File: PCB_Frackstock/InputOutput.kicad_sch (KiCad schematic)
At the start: 30 parts, among them J1 87224-3, U11 CC1101RGPR, U7 BMI323, Y2 26MHz

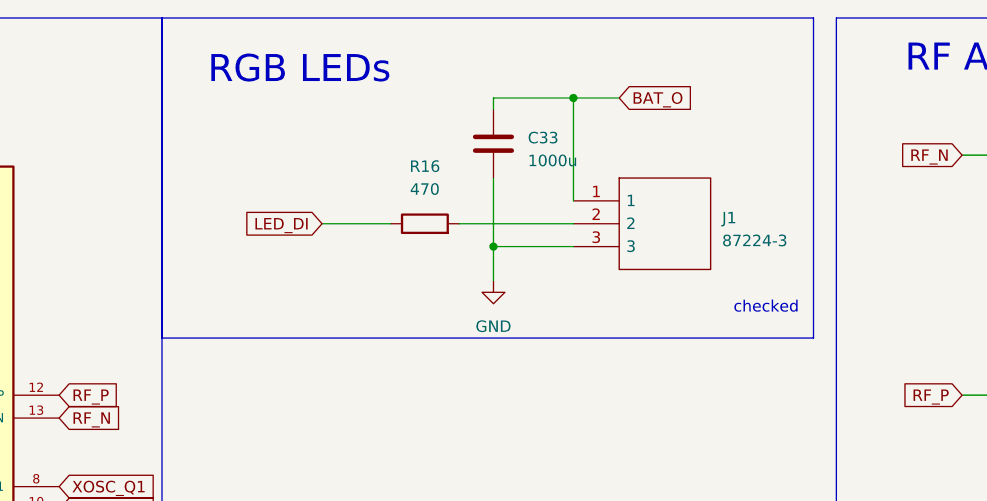
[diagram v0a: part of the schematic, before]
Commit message: Schema_fertig
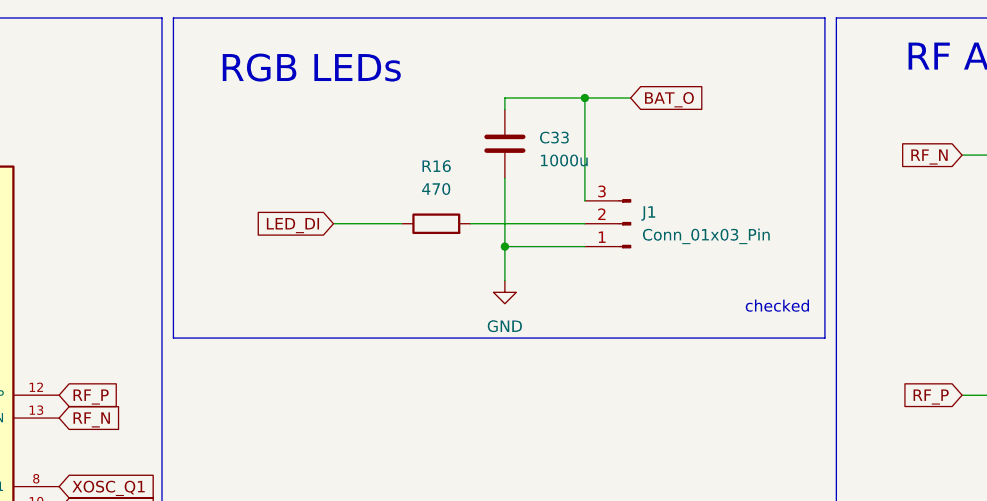
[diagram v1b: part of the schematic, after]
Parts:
- removed J1: 87224-3, KiCad:872243, symbol 87224-3:87224-3
- added J1: Conn_01x03_Pin, Connector_PinHeader_2.54mm:PinHeader_1x03_P2.54mm_Vertical, symbol Connector:Conn_01x03_Pin
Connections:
- net BAT_O: now also J1.3 (Pin_3)
- net GND: now also J1.1 (Pin_1)
- net at R16.2: now also J1.2 (Pin_2)
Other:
- moved on the sheet: C33, R16

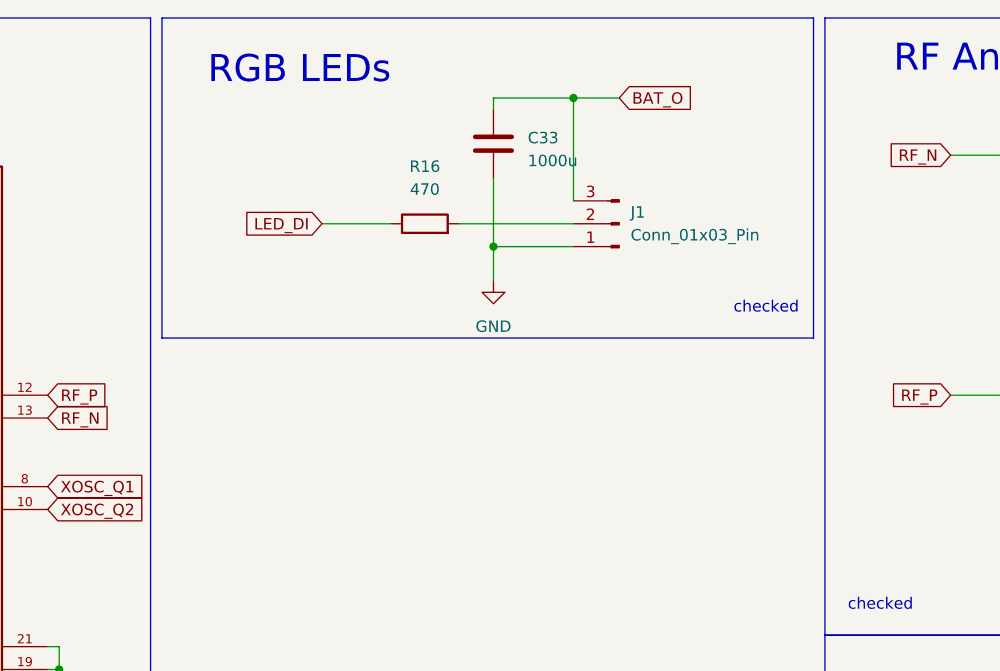
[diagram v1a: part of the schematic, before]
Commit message: Layout Fertig
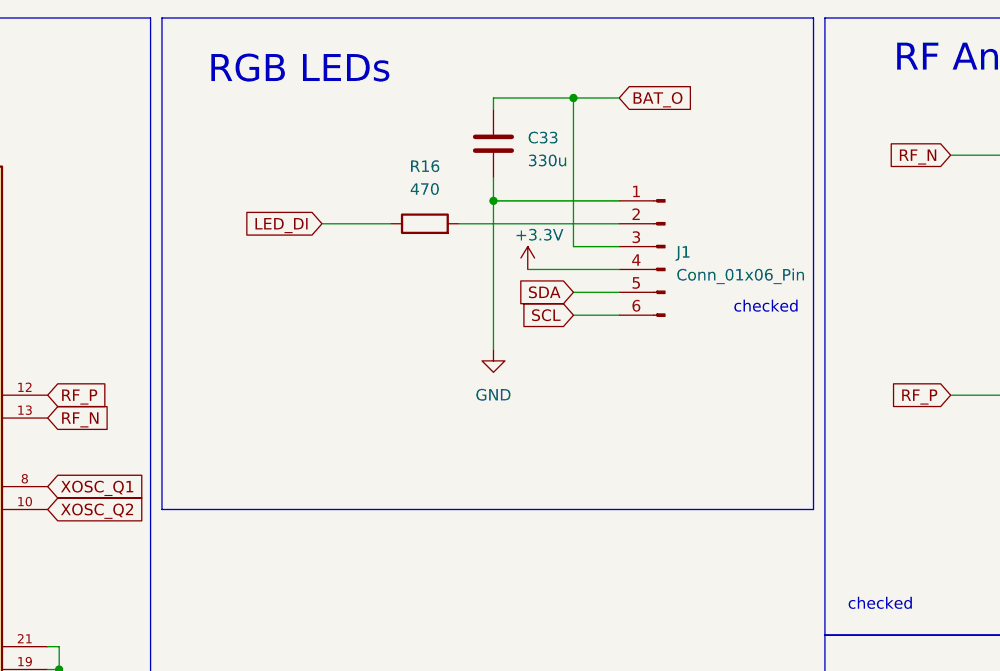
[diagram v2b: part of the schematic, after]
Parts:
- removed J1: Conn_01x03_Pin, Connector_PinHeader_2.54mm:PinHeader_1x03_P2.54mm_Vertical, symbol Connector:Conn_01x03_Pin
- added J1: Conn_01x06_Pin, symbol Connector:Conn_01x06_Pin
- C33: value 1000u -> 330u; footprint Capacitor_SMD:CP_Elec_8x10.5 -> Capacitor_SMD:C_0805_2012Metric_Pad1.18x1.45mm_HandSolder
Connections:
- net +3.3V: now also J1.4 (Pin_4)
- net BAT_O: now also J1.3 (Pin_3)
- net GND: now also J1.1 (Pin_1)
- net at R16.2: now also J1.2 (Pin_2)
- new net SCL: J1.6 (Pin_6)
- new net SDA: J1.5 (Pin_5)
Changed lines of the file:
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@@
   (junction (at 228.6 97.79) (diameter 0) (color 0 0 0 0)
   )
+  (junction (at 134.62 34.29) (diameter 0) (color 0 0 0 0)
+  )
   (junction (at 83.82 177.8) (diameter 0) (color 0 0 0 0)
   )
-  (junction (at 134.62 39.37) (diameter 0) (color 0 0 0 0)
-  )
   (junction (at 240.03 107.95) (diameter 0) (color 0 0 0 0)
   )
@@
     (stroke (width 0) (type default))
   )
+  (wire (pts (xy 143.51 46.99) (xy 148.59 46.99))
+    (stroke (width 0) (type default))
+  )
   (wire (pts (xy 38.1 40.64) (xy 38.1 38.1))
     (stroke (width 0) (type default))
@@
     (stroke (width 0) (type default))
   )
+  (wire (pts (xy 134.62 34.29) (xy 148.59 34.29))
+    (stroke (width 0) (type default))
+  )
+  (wire (pts (xy 134.62 34.29) (xy 134.62 50.8))
+    (stroke (width 0) (type default))
+  )
   (wire (pts (xy 185.42 55.88) (xy 194.31 55.88))
     (stroke (width 0) (type default))
   )
-  (wire (pts (xy 134.62 31.75) (xy 134.62 39.37))
-    (stroke (width 0) (type default))
-  )
   (wire (pts (xy 232.41 41.91) (xy 237.49 41.91))
     (stroke (width 0) (type default))
@@
     (stroke (width 0) (type default))
   )
+  (wire (pts (xy 138.43 41.91) (xy 148.59 41.91))
+    (stroke (width 0) (type default))
+  )
   (wire (pts (xy 134.62 22.86) (xy 134.62 24.13))
     (stroke (width 0) (type default))
@@
     (stroke (width 0) (type default))
   )
-  (wire (pts (xy 130.81 36.83) (xy 143.51 36.83))
+  (wire (pts (xy 130.81 36.83) (xy 148.59 36.83))
     (stroke (width 0) (type default))
   )
@@
     (stroke (width 0) (type default))
   )
-  (wire (pts (xy 134.62 39.37) (xy 134.62 43.18))
+  (wire (pts (xy 134.62 31.75) (xy 134.62 34.29))
     (stroke (width 0) (type default))
   )
@@
     (stroke (width 0) (type default))
   )
+  (wire (pts (xy 143.51 44.45) (xy 148.59 44.45))
+    (stroke (width 0) (type default))
+  )
   (wire (pts (xy 251.46 97.79) (xy 251.46 99.06))
     (stroke (width 0) (type default))
@@
     (stroke (width 0) (type default))
   )
-  (wire (pts (xy 143.51 22.86) (xy 143.51 34.29))
+  (wire (pts (xy 143.51 22.86) (xy 143.51 39.37))
+    (stroke (width 0) (type default))
+  )
+  (wire (pts (xy 143.51 39.37) (xy 148.59 39.37))
     (stroke (width 0) (type default))
   )
@@
     (stroke (width 0) (type default))
   )
-  (wire (pts (xy 134.62 39.37) (xy 143.51 39.37))
-    (stroke (width 0) (type default))
-  )
   (wire (pts (xy 232.41 55.88) (xy 228.6 55.88))
     (stroke (width 0) (type default))
@@
     (stroke (width 0) (type default))
   )
-  (rectangle (start 97.79 13.97) (end 170.18 49.53)
+  (rectangle (start 97.79 13.97) (end 170.18 68.58)
     (stroke (width 0) (type default))
     (fill (type none))
@@
     )
   )
+  (global_label "SDA" (shape input) (at 143.51 44.45 180) (fields_autoplaced)
+    (effects (font (size 1.27 1.27)) (justify right))
+    (property "Intersheetrefs" "${INTERSHEET_REFS}" (at 137.0361 44.45 0)
+      (effects (font (size 1.27 1.27)) (justify right) hide)
+    )
+  )
   (global_label "RF_P" (shape input) (at 185.42 55.88 180) (fields_autoplaced)
     (effects (font (size 1.27 1.27)) (justify right))
@@
     )
   )
+  (global_label "SCL" (shape input) (at 143.51 46.99 180) (fields_autoplaced)
+    (effects (font (size 1.27 1.27)) (justify right))
+    (property "Intersheetrefs" "${INTERSHEET_REFS}" (at 137.0966 46.99 0)
+      (effects (font (size 1.27 1.27)) (justify right) hide)
+    )
+  )
   (global_label "XOSC_Q2" (shape input) (at 85.09 68.58 0) (fields_autoplaced)
     (effects (font (size 1.27 1.27)) (justify left))
@@
         (path "/d92252e1-c687-49e6-87c8-e9430a2c933e/c15a2309-71af-495b-84ee-43442cf95a1c"
           (reference "#PWR019") (unit 1)
+        )
+      )
+    )
+  )
+  (symbol (lib_id "power:+3.3V") (at 138.43 41.91 0) (unit 1)
+    (in_bom yes) (on_board yes) (dnp no)
+    (property "Reference" "#PWR03" (at 138.43 45.72 0)
+      (effects (font (size 1.27 1.27)) hide)
+    )
+    (property "Value" "+3.3V" (at 139.7 38.1 0)
+      (effects (font (size 1.27 1.27)))
+    )
+    (property "Footprint" "" (at 138.43 41.91 0)
+      (effects (font (size 1.27 1.27)) hide)
+    )
+    (property "Datasheet" "" (at 138.43 41.91 0)
+      (effects (font (size 1.27 1.27)) hide)
+    )
+    (pin "1")
+    (instances
+      (project "Frackstock"
+        (path "/d92252e1-c687-49e6-87c8-e9430a2c933e/c15a2309-71af-495b-84ee-43442cf95a1c"
+          (reference "#PWR03") (unit 1)
         )
       )
@@
     )
   )
-  (symbol (lib_id "power:GND") (at 134.62 43.18 0) (unit 1)
-    (in_bom yes) (on_board yes) (dnp no) (fields_autoplaced)
-    (property "Reference" "#PWR013" (at 134.62 49.53 0)
-      (effects (font (size 1.27 1.27)) hide)
-    )
-    (property "Value" "GND" (at 134.62 48.26 0)
-      (effects (font (size 1.27 1.27)))
-    )
-    (property "Footprint" "" (at 134.62 43.18 0)
-      (effects (font (size 1.27 1.27)) hide)
-    )
-    (property "Datasheet" "" (at 134.62 43.18 0)
+  (symbol (lib_id "power:GND") (at 134.62 50.8 0) (unit 1)
+    (in_bom yes) (on_board yes) (dnp no) (fields_autoplaced)
+    (property "Reference" "#PWR013" (at 134.62 57.15 0)
+      (effects (font (size 1.27 1.27)) hide)
+    )
+    (property "Value" "GND" (at 134.62 55.88 0)
+      (effects (font (size 1.27 1.27)))
+    )
+    (property "Footprint" "" (at 134.62 50.8 0)
+      (effects (font (size 1.27 1.27)) hide)
+    )
+    (property "Datasheet" "" (at 134.62 50.8 0)
       (effects (font (size 1.27 1.27)) hide)
     )
@@
       (effects (font (size 1.27 1.27)) (justify right))
     )
-    (property "Value" "1000u" (at 138.43 29.845 0)
+    (property "Value" "330u" (at 138.43 29.845 0)
       (effects (font (size 1.27 1.27)) (justify right))
     )
-    (property "Footprint" "Capacitor_SMD:CP_Elec_8x10.5" (at 133.6548 24.13 0)
+    (property "Footprint" "Capacitor_SMD:C_0805_2012Metric_Pad1.18x1.45mm_HandSolder" (at 133.6548 24.13 0)
       (effects (font (size 1.27 1.27)) hide)
     )
@@
         (path "/d92252e1-c687-49e6-87c8-e9430a2c933e/c15a2309-71af-495b-84ee-43442cf95a1c"
           (reference "C37") (unit 1)
+        )
+      )
+    )
+  )
+  (symbol (lib_id "Connector:Conn_01x06_Pin") (at 153.67 39.37 0) (mirror y) (unit 1)
+    (in_bom yes) (on_board yes) (dnp no) (fields_autoplaced)
+    (property "Reference" "J1" (at 154.94 40.005 0)
+      (effects (font (size 1.27 1.27)) (justify right))
+    )
+    (property "Value" "Conn_01x06_Pin" (at 154.94 42.545 0)
+      (effects (font (size 1.27 1.27)) (justify right))
+    )
+    (property "Footprint" "" (at 153.67 39.37 0)
+      (effects (font (size 1.27 1.27)) hide)
+    )
+    (property "Datasheet" "~" (at 153.67 39.37 0)
+      (effects (font (size 1.27 1.27)) hide)
+    )
+    (pin "1")
+    (pin "2")
+    (pin "3")
+    (pin "4")
+    (pin "5")
+    (pin "6")
+    (instances
+      (project "Frackstock"
+        (path "/d92252e1-c687-49e6-87c8-e9430a2c933e/c15a2309-71af-495b-84ee-43442cf95a1c"
+          (reference "J1") (unit 1)
         )
       )
@@
         )
       )
-    )
-  )
-  (symbol (lib_id "Connector:Conn_01x03_Pin") (at 148.59 36.83 180) (unit 1)
-    (in_bom yes) (on_board yes) (dnp no) (fields_autoplaced)
-    (property "Reference" "J1" (at 149.86 35.56 0)
-      (effects (font (size 1.27 1.27)) (justify right))
-    )
-    (property "Value" "Conn_01x03_Pin" (at 149.86 38.1 0)
-      (effects (font (size 1.27 1.27)) (justify right))
-    )
-    (property "Footprint" "Connector_PinHeader_2.54mm:PinHeader_1x03_P2.54mm_Vertical" (at 148.59 36.83 0)
-      (effects (font (size 1.27 1.27)) hide)
-    )
-    (property "Datasheet" "~" (at 148.59 36.83 0)
-      (effects (font (size 1.27 1.27)) hide)
-    )
-    (pin "1")
-    (pin "2")
-    (pin "3")
-    (instances
-      (project "Frackstock"
-        (path "/d92252e1-c687-49e6-87c8-e9430a2c933e/c15a2309-71af-495b-84ee-43442cf95a1c"
-          (reference "J1") (unit 1)
-        )
-      )

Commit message: Layout Update
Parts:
- J1: footprint (none) -> Frack:PinHeader_2x03_P2.54mm_Vertical_SMD_kleiner
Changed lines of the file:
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@@
       (effects (font (size 1.27 1.27)) (justify right))
     )
-    (property "Footprint" "" (at 153.67 39.37 0)
+    (property "Footprint" "Frack:PinHeader_2x03_P2.54mm_Vertical_SMD_kleiner" (at 153.67 39.37 0)
       (effects (font (size 1.27 1.27)) hide)
     )
